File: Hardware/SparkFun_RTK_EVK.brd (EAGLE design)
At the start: 165.5 x 131.1 mm, 440 parts, among them J3 MICRO-SD-PUSH-PUSH-EXT-PIN, J4 Vertical Qwiic Connector, J9 MAGJACK-POE, Q5 310mA/60V/1.6Ω, Q6 310mA/60V/1.6Ω, U1 ESP32-WROVER-IE, U10 POE_PSU-DP990X, U11 MCP6021T, U12 AP7361C-33, U13 MCP6021T, U14 BP2G1+_POWER_SPLITTER, U15 USB251XB_USB2514B, U16 SN74AVC4T774PW, U17 URB2405YMD, U18 74HC1G04, U2 CH340C, U3 XC6222B331MR-G, U4 U-BLOX_ZED-F9P, U5 U-BLOX_NEO-D9S-00B, U6 XC6222B331MR-G, U7 W5500, U8 LARA-R6001D, U9 74LVC4066D_QUAD_BILATERAL_SWI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, Y1 25MHz, Y2 24MHz

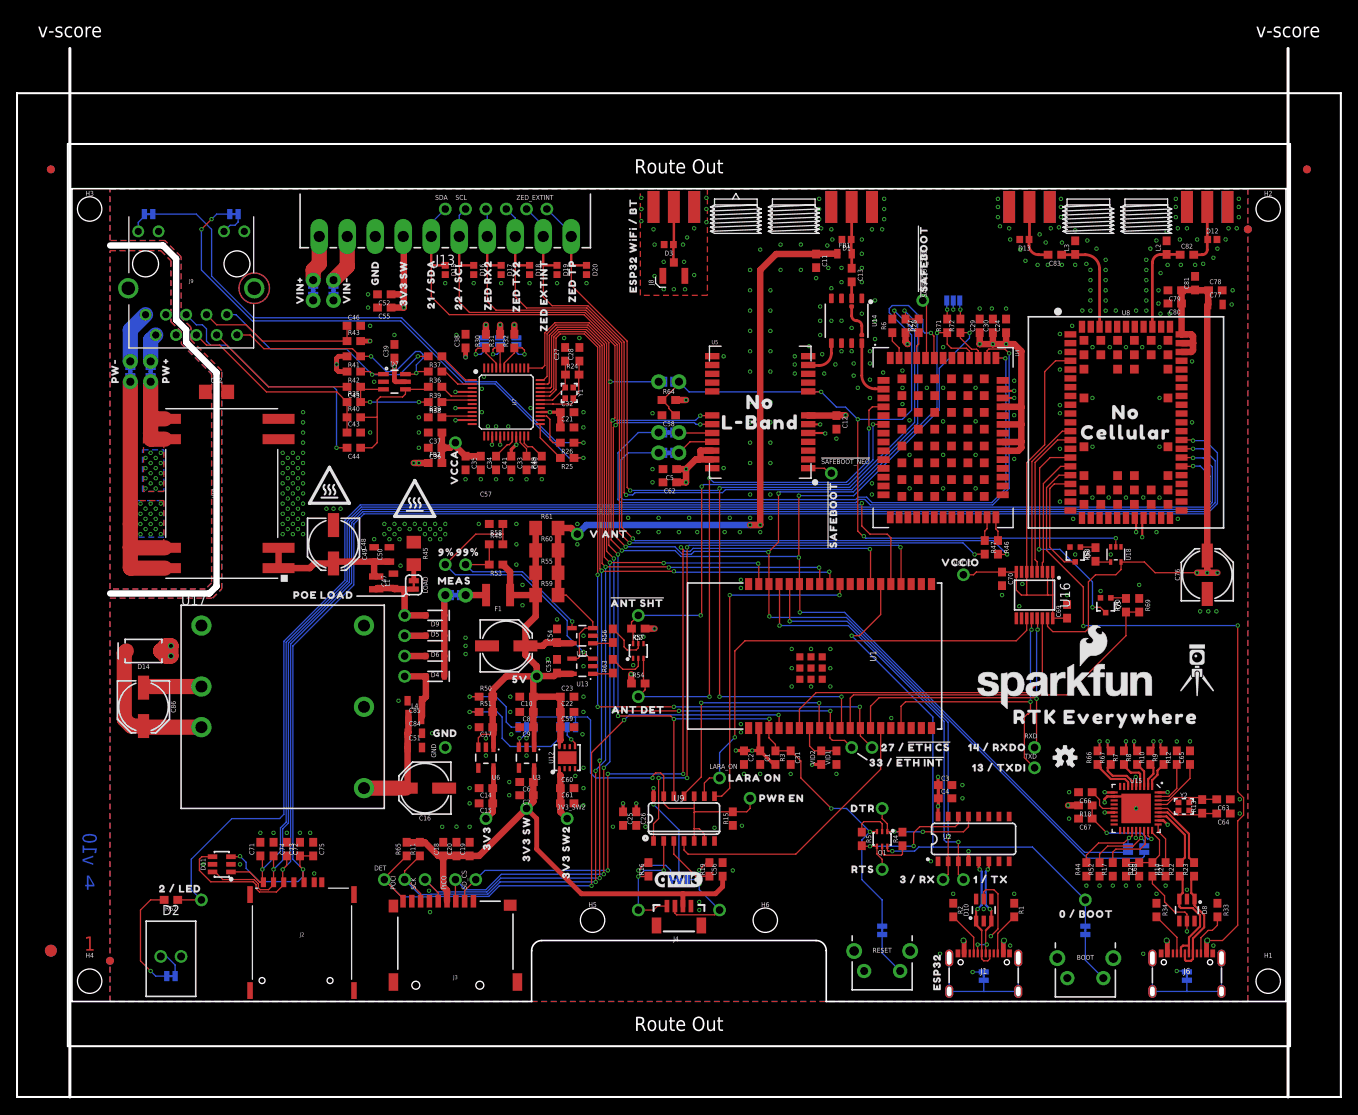
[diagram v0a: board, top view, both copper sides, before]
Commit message: v11 PCB
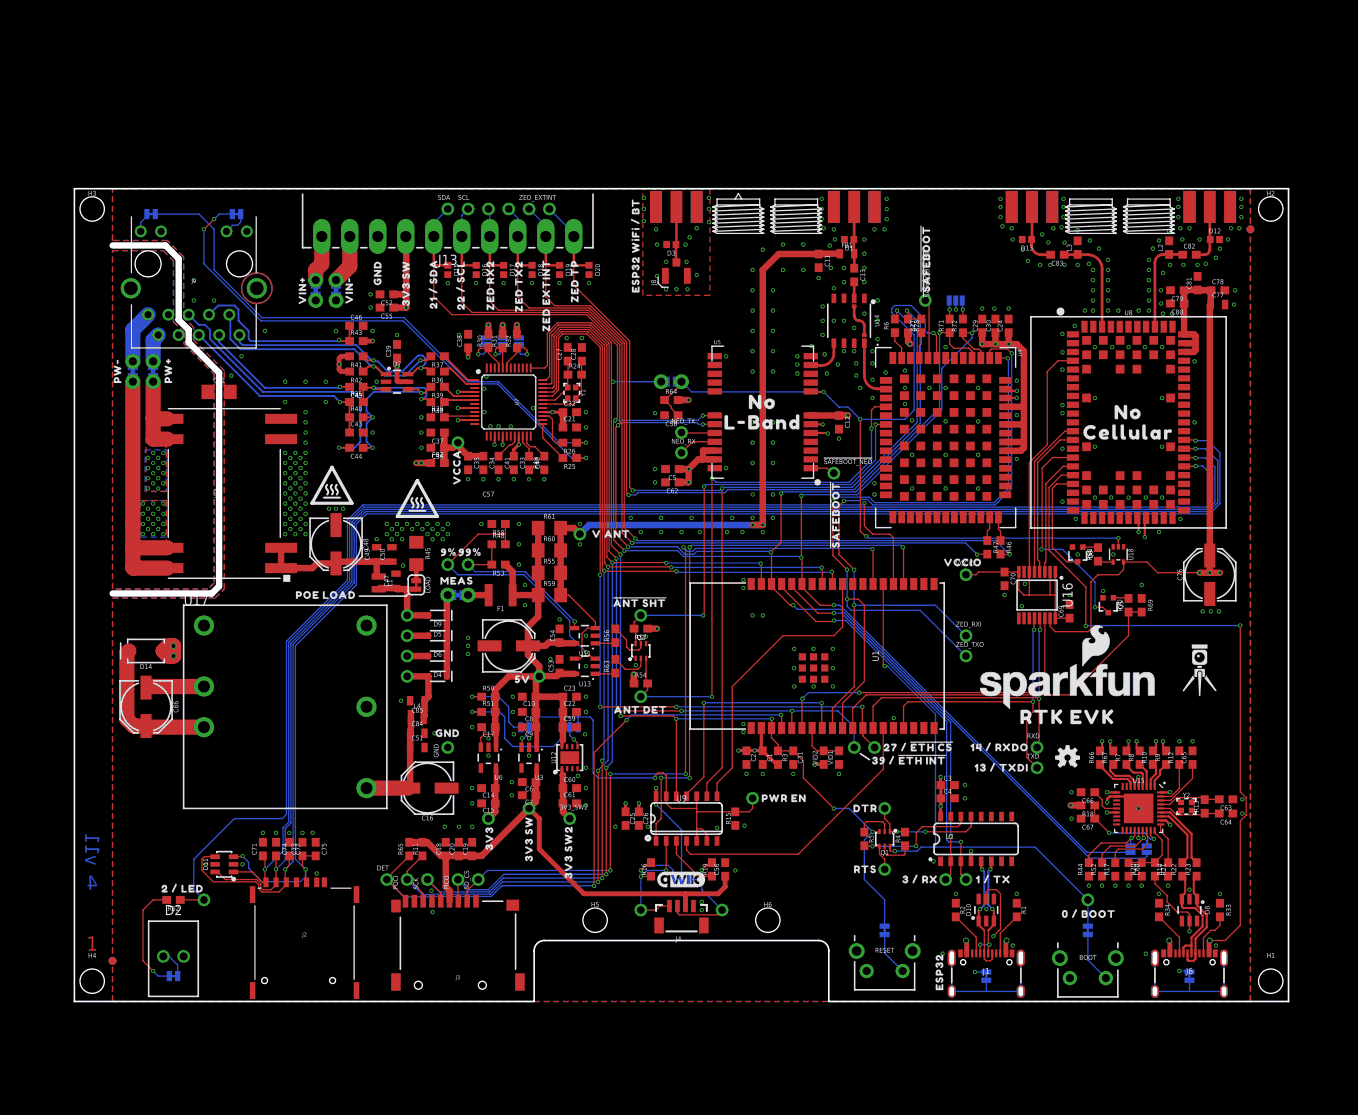
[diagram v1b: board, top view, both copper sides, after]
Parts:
- removed E$1, E$2, E$3, E$4: (no value), SparkFun-Aesthetics:FIDUCIAL-1X2
- removed E$5, E$6: (no value), SparkFun-Retired:FIDUCIAL-1.5X3
- removed LARA_ON: TEST-POINTPOGO_PTH, SparkFun-Connectors:1X01_NO_SILK
- removed RX-TX, TX-RX: JUMPER-COMBO_2_NC_TRACE, SparkFun-Jumpers:COMBO-JUMPER_2_NC_TRACE
- removed U$109, U$27: (no value), output:33_#_#ETH_INT#0
- removed U$112: (no value), output:LARA_ON0
- added FRAME1: FRAME-LEDGER, SparkFun-Aesthetics:CREATIVE_COMMONS
- added FRAME2: FRAME-LEDGERNO_FOOTPRINT, SparkFun-Aesthetics:DUMMY
- added LOGO1: SPECIAL_INSTRUCTIONS-ORDERING, SparkFun-Aesthetics:ORDERING_INSTRUCTIONS
- added NEO_RX, NEO_TX, ZED_RXI, ZED_TXO: TEST-POINTPOGO_PTH, SparkFun-Connectors:1X01_NO_SILK
- U$11: device output:ZED_TX1 -> output:RTK_EVK0
- U$110: device output:LARA_ON0 -> output:39_#_#ETH_INT#0
- U$13: device output:ZED_RX0 -> output:RTK_EVK0
- U$2: device output:RTK_EVERYWHERE0 -> output:33_#_ZED_RXI0
- U$79: device output:UART14 -> output:39_#_#ETH_INT#0
- U$90: device output:RTK_EVERYWHERE0 -> output:25_#_ZED_TXO0
- moved U$11 64.1 mm to (124.5, 35.6), flipped to the top
- moved U$13 61.4 mm to (130.8, 67.3)
- moved U$79 49.3 mm to (99.3, 30.2), flipped to the top
- moved U$90 27.9 mm to (111.4, 43.2)
- moved U$2 20.5 mm to (111.4, 45.7), flipped to the bottom
- moved U$110 16.7 mm to (97.5, 31.9), flipped to the bottom
- moved C68 0.32 mm to (132.1, 16.5)
- moved H1 0.32 mm to (149.9, 2.54)
- moved H2 0.32 mm to (149.9, 99.1)
- moved R67 0.32 mm to (130.2, 30.5)
- moved R70 0.32 mm to (132.1, 49.5)
- moved U$92 0.32 mm to (132.1, 73.7)
- moved U$96 0.32 mm to (132.1, 71.1)
- moved U8 0.32 mm to (132.1, 72.4)
- moved USB251SCL 0.32 mm to (134.4, 19.1)
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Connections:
- net ESP5/LARA_ON renamed ESP5/TP
- removed net ESP25/TP: D20.1, J13.1, R6.2, TP.1, U1.10
- removed net ESP33/!ETH_INT!: ETH_INT.1, U1.9, U7.36
- removed net LARA_ON: LARA_ON.1, U16.11, U9.9
- removed net ZED_RXI: RX-TX.2, RX-TX.4, U4.43
- removed net ZED_TXO: TX-RX.1, TX-RX.3, U4.42
- new net ESP25/ZED_TXO: U1.10, U4.42, ZED_TXO.1
- new net ESP33/ZED_RXI: U1.9, U4.43, ZED_RXI.1
- new net ESP39/!ETH_INT!: ETH_INT.1, U1.5, U7.36
- new net ZED_TP: D20.1, J13.1, R6.2, TP.1, U9.9
- net NEO_RXI: now also NEO_RX.1; no longer TX-RX.2, TX-RX.4
- net NEO_TXO: now also NEO_TX.1; no longer RX-TX.1, RX-TX.3
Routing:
- net ESP25/TP: track 141.9 -> 0.00 mm, vias 5 -> 0
- net ZED_TP: track 0.00 -> 135.9 mm, vias 0 -> 3
- net ESP39/!ETH_INT!: track 0.00 -> 96.8 mm, vias 0 -> 4
- net ESP33/!ETH_INT!: track 95.2 -> 0.00 mm, vias 4 -> 0
- net ESP25/ZED_TXO: track 0.00 -> 90.9 mm, vias 0 -> 4
- net ESP33/ZED_RXI: track 0.00 -> 89.2 mm, vias 0 -> 4
- net ZED_RXI: track 84.0 -> 0.00 mm, vias 1 -> 0
- net ZED_TXO: track 77.4 -> 0.00 mm, vias 1 -> 0
- net LARA_ON: track 59.5 -> 0.00 mm, vias 1 -> 0
- net ESP5/TP: track 41.6 -> 36.7 mm, vias 2 -> 0
- net RD-: track 32.1 -> 36.1 mm
- net ESP0/!BOOT!: track 70.7 -> 67.3 mm
- net RXN1: track 17.2 -> 20.0 mm, vias 0 -> 3
- net VCCA: track 69.6 -> 72.3 mm
- net CH340-RXI: track 52.4 -> 49.7 mm
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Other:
- board size 165.5 x 131.1 mm -> 151.8 x 101.6 mm
- board text added: "Controlled Impedance: JLC7628 Material: TG155 4-Layers Thickness: 1.6mm Outer Copper: 1oz Inner Copper: 0.5oz Finish: HASL Lead Free Red Solder Resist White Silkscreen"
- board text added: "Dimensions In Inches"
- board text added: "Paul Clark"
- board text added: "V-Score To V-Score"
- board text added: "v11"
- board text removed: "Route Out"
- board text removed: "v-score"
- board text removed: "v10"
